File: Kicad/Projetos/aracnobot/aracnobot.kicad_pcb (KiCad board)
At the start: 2 copper layers, 1 part, among them U1 RASPBERRY_PI_3_MODEL_B_

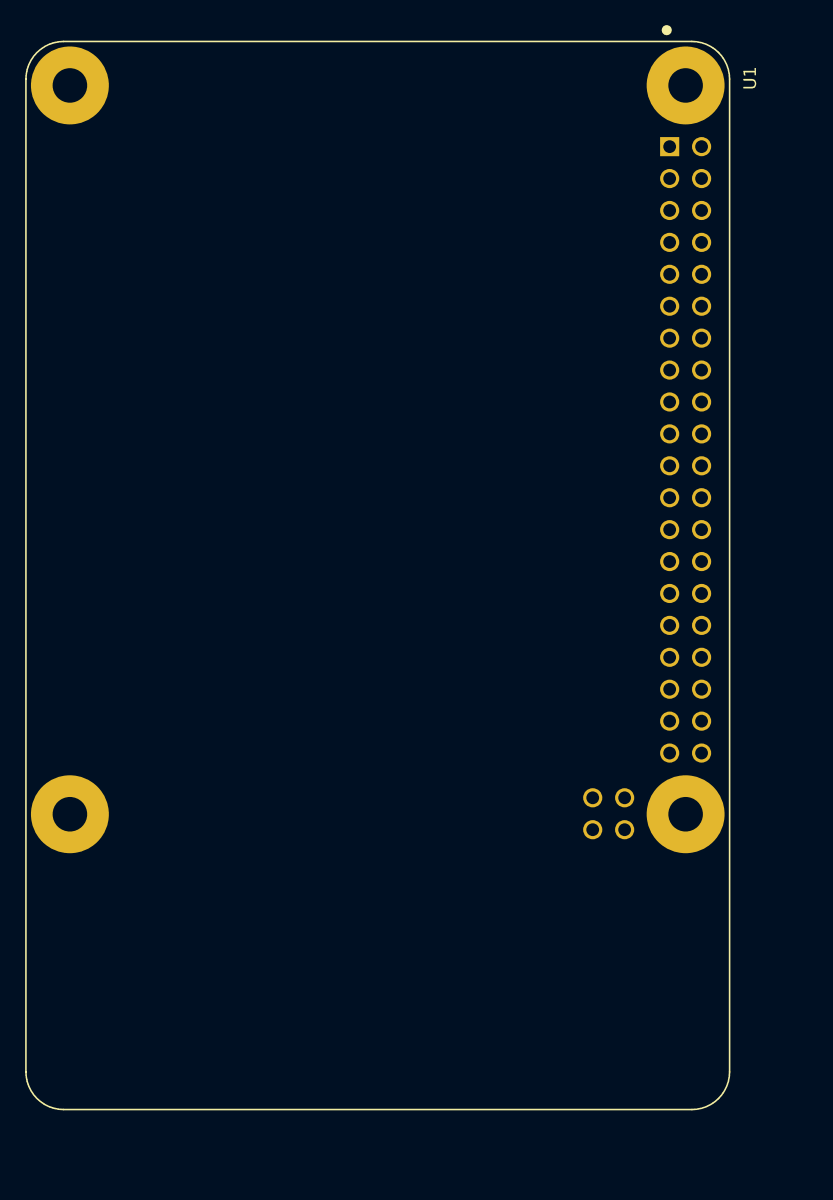
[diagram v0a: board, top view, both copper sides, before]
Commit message: model 4 B
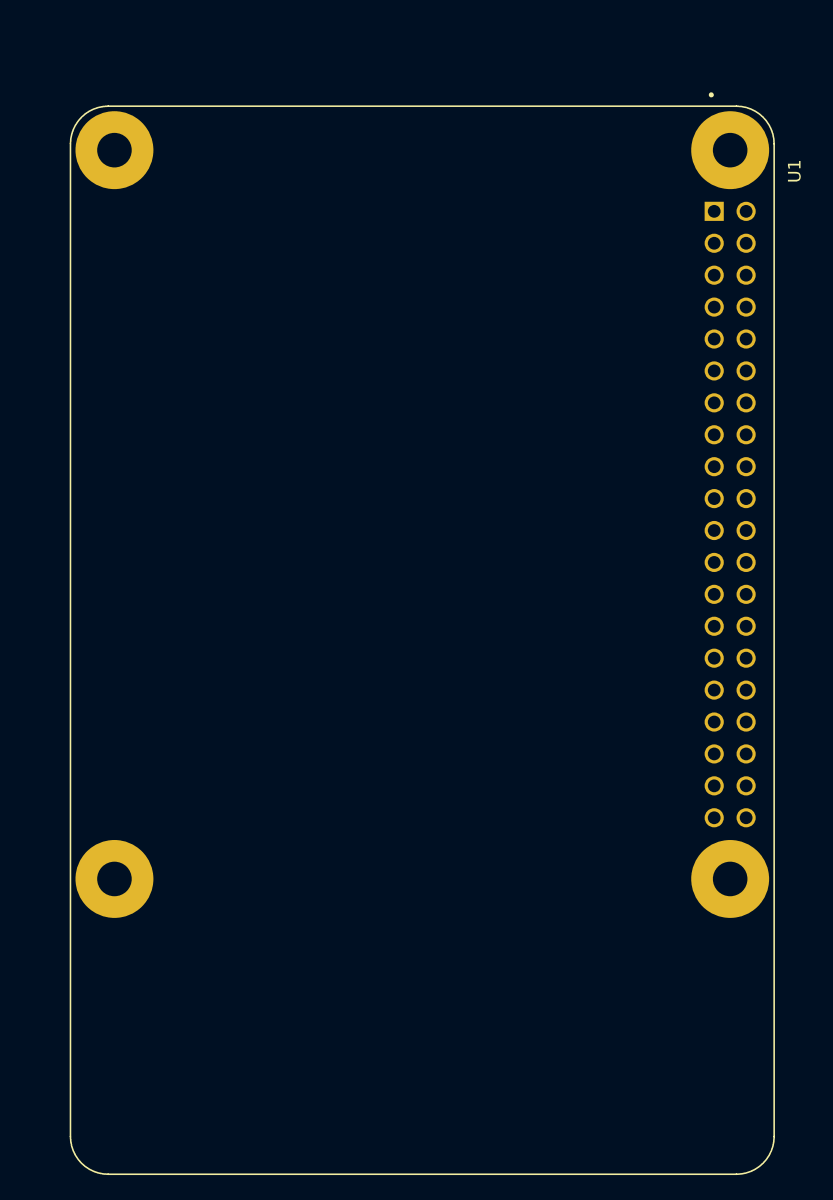
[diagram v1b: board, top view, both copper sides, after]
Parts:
- U1: value RASPBERRY_PI_3_MODEL_B_ -> SC0195_9_; footprint Raspberry_Pi_Footprints:MODULE_RASPBERRY_PI_3_MODEL_B_ -> Raspberry_pi_4_B:MODULE_SRASPBERRY_PI_4_MODEL_B_
- moved U1 6.25 mm to (53.3, 100.0)
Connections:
- net 5V renamed 5V0
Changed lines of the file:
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@@
 		)
 	)
-	(footprint "Raspberry_Pi_Footprints:MODULE_RASPBERRY_PI_3_MODEL_B_"
+	(footprint "Raspberry_pi_4_B:MODULE_SRASPBERRY_PI_4_MODEL_B_"
 		(layer "F.Cu")
-		(at 49.725 94.8 -90)
+		(at 53.27 99.95 -90)
 		(property "Reference" "U1"
-			(at -39.575 -29.635 90)
-			(layer "F.SilkS")
-			(effects
-				(font
-					(size 1 1)
-					(thickness 0.15)
-				)
-			)
-		)
-		(property "Value" "RASPBERRY_PI_3_MODEL_B_"
-			(at -23.7 31.135 90)
+			(at -37.325 -29.635 90)
+			(layer "F.SilkS")
+			(effects
+				(font
+					(size 1 1)
+					(thickness 0.15)
+				)
+			)
+		)
+		(property "Value" "SC0195_9_"
+			(at -30.54 29.965 90)
 			(layer "F.Fab")
 			(effects
@@
 			)
 		)
-		(property "Description" "Single Board Computer, Model B+ 1GB RAM,Raspberry Pi 3 Series | Raspberry Pi RASPBERRY PI 3 MODEL B+"
+		(property "Description" "The Raspberry Pi 4 Model B SC0195-9 single board computer features a powerful Broadcom BCM2711 ARM Cortex-A72 processor with 1.5GHz speed and four cores, making it ideal for demanding embedded computing applications. With 8GB of RAM and a compact size of 3.346 x 2.205, this SBC offers robust performance in a small footprint. It includes 40 digital I/O lines, GbE Ethernet, and multiple USB ports (two USB 2.0 and two USB 3.0), providing versatile connectivity options. Additionally, it supports video outputs such as CSI, DSI, and HDMI, making it suitable for a wide range of multimedia projects."
 			(at 0 0 90)
 			(layer "F.Fab")
@@
 			)
 		)
-		(property "MAXIMUM_PACKAGE_HEIGHT" "16 mm"
-			(at 0 0 270)
-			(unlocked yes)
-			(layer "F.Fab")
-			(hide yes)
-			(effects
-				(font
-					(size 1 1)
-					(thickness 0.15)
-				)
-			)
-		)
-		(property "Package" "Raspberry Pi"
+		(property "Package" "None"
 			(at 0 0 270)
 			(unlocked yes)
@@
 			)
 		)
-		(property "Check_prices" "https://www.snapeda.com/parts/RASPBERRY%20PI%203%20MODEL%20B+/Raspberry+Pi/view-part/?ref=eda"
+		(property "Check_prices" "https://www.snapeda.com/parts/SC0195(9)/Raspberry+Pi/view-part/?ref=eda"
+			(at 0 0 270)
+			(unlocked yes)
+			(layer "F.Fab")
+			(hide yes)
+			(effects
+				(font
+					(size 1 1)
+					(thickness 0.15)
+				)
+			)
+		)
+		(property "MAXIMUM_PACKAGE_HIEGHT" "18mm"
 			(at 0 0 270)
 			(unlocked yes)
@@
 			)
 		)
-		(property "PARTREV" "N/A"
-			(at 0 0 270)
-			(unlocked yes)
-			(layer "F.Fab")
-			(hide yes)
-			(effects
-				(font
-					(size 1 1)
-					(thickness 0.15)
-				)
-			)
-		)
-		(property "SnapEDA_Link" "https://www.snapeda.com/parts/RASPBERRY%20PI%203%20MODEL%20B+/Raspberry+Pi/view-part/?ref=snap"
-			(at 0 0 270)
-			(unlocked yes)
-			(layer "F.Fab")
-			(hide yes)
-			(effects
-				(font
-					(size 1 1)
-					(thickness 0.15)
-				)
-			)
-		)
-		(property "MP" "RASPBERRY PI 3 MODEL B+"
-			(at 0 0 270)
-			(unlocked yes)
-			(layer "F.Fab")
-			(hide yes)
-			(effects
-				(font
-					(size 1 1)
-					(thickness 0.15)
-				)
-			)
-		)
-		(property "SNAPEDA_PN" "RASPBERRY PI 3 MODEL B+"
+		(property "PARTREV" "1.0"
+			(at 0 0 270)
+			(unlocked yes)
+			(layer "F.Fab")
+			(hide yes)
+			(effects
+				(font
+					(size 1 1)
+					(thickness 0.15)
+				)
+			)
+		)
+		(property "SnapEDA_Link" "https://www.snapeda.com/parts/SC0195(9)/Raspberry+Pi/view-part/?ref=snap"
+			(at 0 0 270)
+			(unlocked yes)
+			(layer "F.Fab")
+			(hide yes)
+			(effects
+				(font
+					(size 1 1)
+					(thickness 0.15)
+				)
+			)
+		)
+		(property "MP" "SC0195(9)"
 			(at 0 0 270)
 			(unlocked yes)
@@
 				(name "A")
 				(pins "3" "5" "7" "11" "13" "12" "15" "16" "18" "22" "24" "26" "23" "19"
-					"21" "27" "28" "2" "4" "1" "17" "8" "10" "29" "31" "32" "33" "36" "35"
-					"38" "40" "37" "42" "41" "44" "43" "S4" "S3" "S2" "S1" "39" "34" "30"
-					"25" "20" "14" "9" "6"
+					"21" "27" "28" "2" "4" "17" "1" "8" "10" "29" "31" "32" "33" "36" "35"
+					"38" "40" "37" "S2" "S1" "S3" "S4" "34" "30" "39" "6" "25" "9" "14"
+					"20"
 				)
 			)
@@
 		(fp_circle
 			(center -43.4 -23)
-			(end -43.2 -23)
-			(stroke
-				(width 0.4)
+			(end -43.3 -23)
+			(stroke
+				(width 0.2)
 				(type solid)
 			)
@@
 		)
 		(fp_line
-			(start -42.75 30.255)
+			(start -42.75 30.75)
 			(end -42.75 -28.25)
 			(stroke
@@
 		)
 		(fp_line
-			(start 45.25 30.255)
-			(end -42.75 30.255)
+			(start 45.25 30.75)
+			(end -42.75 30.75)
 			(stroke
 				(width 0.05)
@@
 		(fp_line
 			(start 45.25 -28.25)
-			(end 45.25 30.255)
+			(end 45.25 30.75)
 			(stroke
 				(width 0.05)
@@
 		(fp_circle
 			(center -43.4 -23)
-			(end -43.2 -23)
-			(stroke
-				(width 0.4)
+			(end -43.3 -23)
+			(stroke
+				(width 0.2)
 				(type solid)
 			)
@@
 			(layers "*.Cu" "*.Mask")
 			(remove_unused_layers no)
-			(net "5V")
-			(pinfunction "5V_2")
+			(net "5V0")
+			(pinfunction "5V0_2")
 			(pintype "power_in")
 			(solder_mask_margin 0.102)
@@
 			(layers "*.Cu" "*.Mask")
 			(remove_unused_layers no)
-			(net "5V")
-			(pinfunction "5V_4")
+			(net "5V0")
+			(pinfunction "5V0_4")
 			(pintype "power_in")
 			(solder_mask_margin 0.102)
@@
 			(layers "*.Cu" "*.Mask")
 			(remove_unused_layers no)
-			(net "unconnected-(U1-GPIO14{slash}TXD0-Pad8)")
-			(pinfunction "GPIO14/TXD0_8")
+			(net "unconnected-(U1-TXD0{slash}GPIO14-Pad8)")
+			(pinfunction "TXD0/GPIO14_8")
 			(pintype "bidirectional")
 			(solder_mask_margin 0.102)
@@
 			(layers "*.Cu" "*.Mask")
 			(remove_unused_layers no)
-			(net "unconnected-(U1-GPIO15{slash}RXD0-Pad10)")
-			(pinfunction "GPIO15/RXD0_10")
+			(net "unconnected-(U1-RXD0{slash}GPIO15-Pad10)")
+			(pinfunction "RXD0/GPIO15_10")
 			(pintype "bidirectional")
 			(solder_mask_margin 0.102)
@@
 			(pintype "bidirectional")
 			(solder_mask_margin 0.102)
-		)
-		(pad "41" thru_hole circle
-			(at 20.23 -17.107 270)
-			(size 1.524 1.524)
-			(drill 1.016)
-			(layers "*.Cu" "*.Mask")
-			(remove_unused_layers no)
-			(net "unconnected-(U1-TR01-Pad41)")
-			(pinfunction "TR01_41")
-			(pintype "bidirectional")
-			(solder_mask_margin 0.102)
-		)
-		(pad "42" thru_hole circle
-			(at 20.23 -19.647 270)
-			(size 1.524 1.524)
-			(drill 1.016)
-			(layers "*.Cu" "*.Mask")
-			(remove_unused_layers no)
-			(net "unconnected-(U1-TR00-Pad42)")
-			(pinfunction "TR00_42")
-			(pintype "bidirectional")
-			(solder_mask_margin 0.102)
-		)
-		(pad "43" thru_hole circle
-			(at 17.69 -17.107 270)
-			(size 1.524 1.524)
-			(drill 1.016)
-			(layers "*.Cu" "*.Mask")
-			(remove_unused_layers no)
-			(net "unconnected-(U1-TR03-Pad43)")
-			(pinfunction "TR03_43")
-			(pintype "bidirectional")
-			(solder_mask_margin 0.102)
-		)
-		(pad "44" thru_hole circle
-			(at 17.69 -19.647 270)
-			(size 1.524 1.524)
-			(drill 1.016)
-			(layers "*.Cu" "*.Mask")
-			(remove_unused_layers no)
-			(net "unconnected-(U1-TR02-Pad44)")
-			(pinfunction "TR02_44")
-			(pintype "bidirectional")
-			(solder_mask_margin 0.102)
